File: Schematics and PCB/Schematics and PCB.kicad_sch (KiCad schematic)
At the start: 3 parts, among them J1 Magnetic Left, J2 Magnetic Right, U1 SN74AUC1G126DBVR

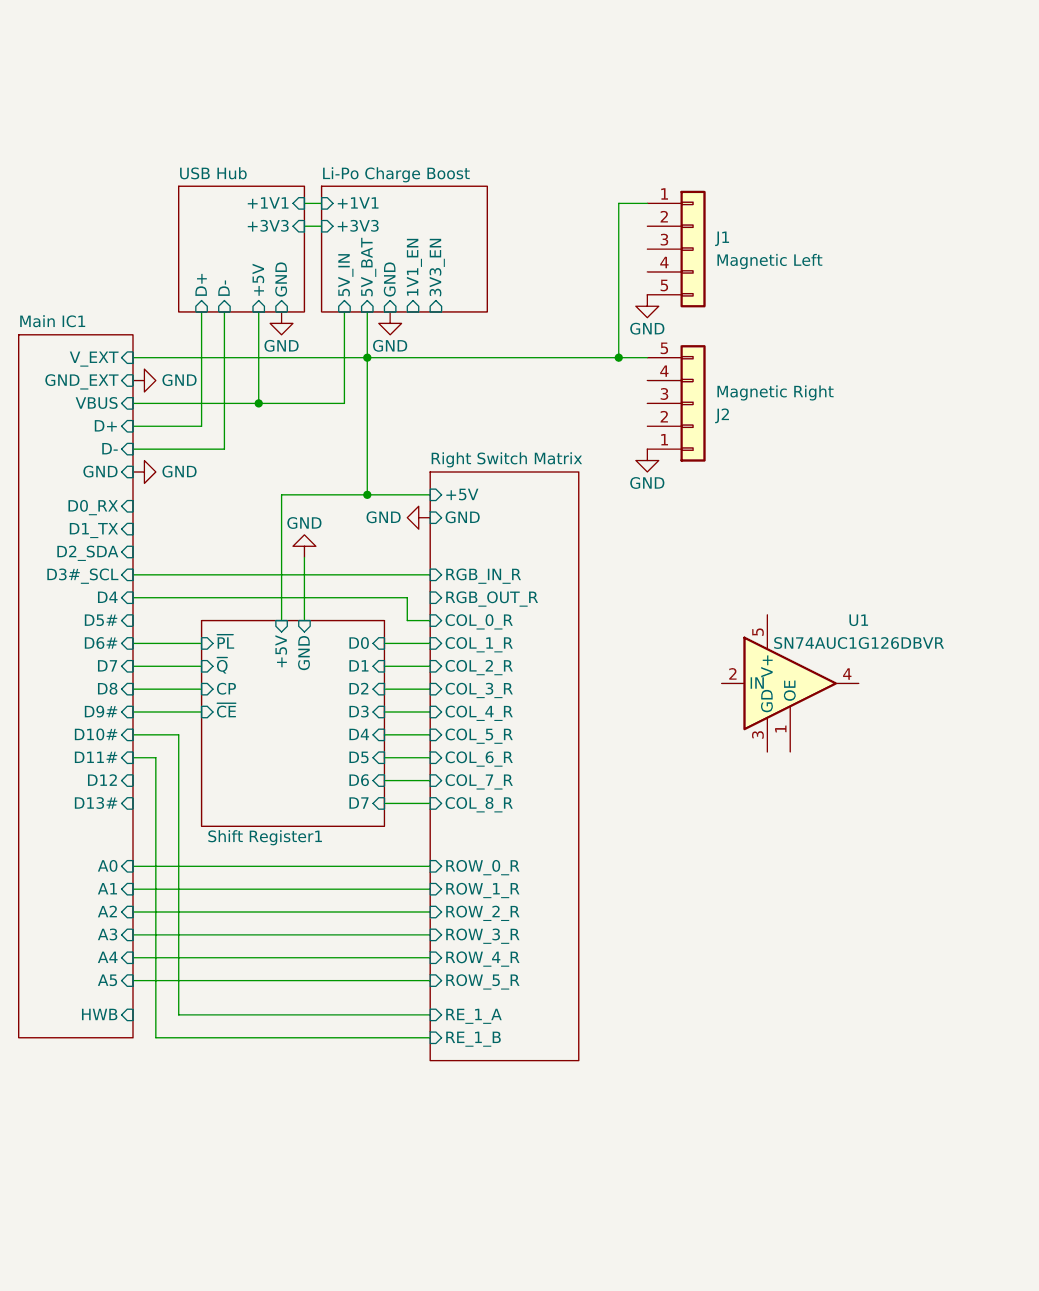
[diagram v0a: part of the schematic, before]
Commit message: Right layout created
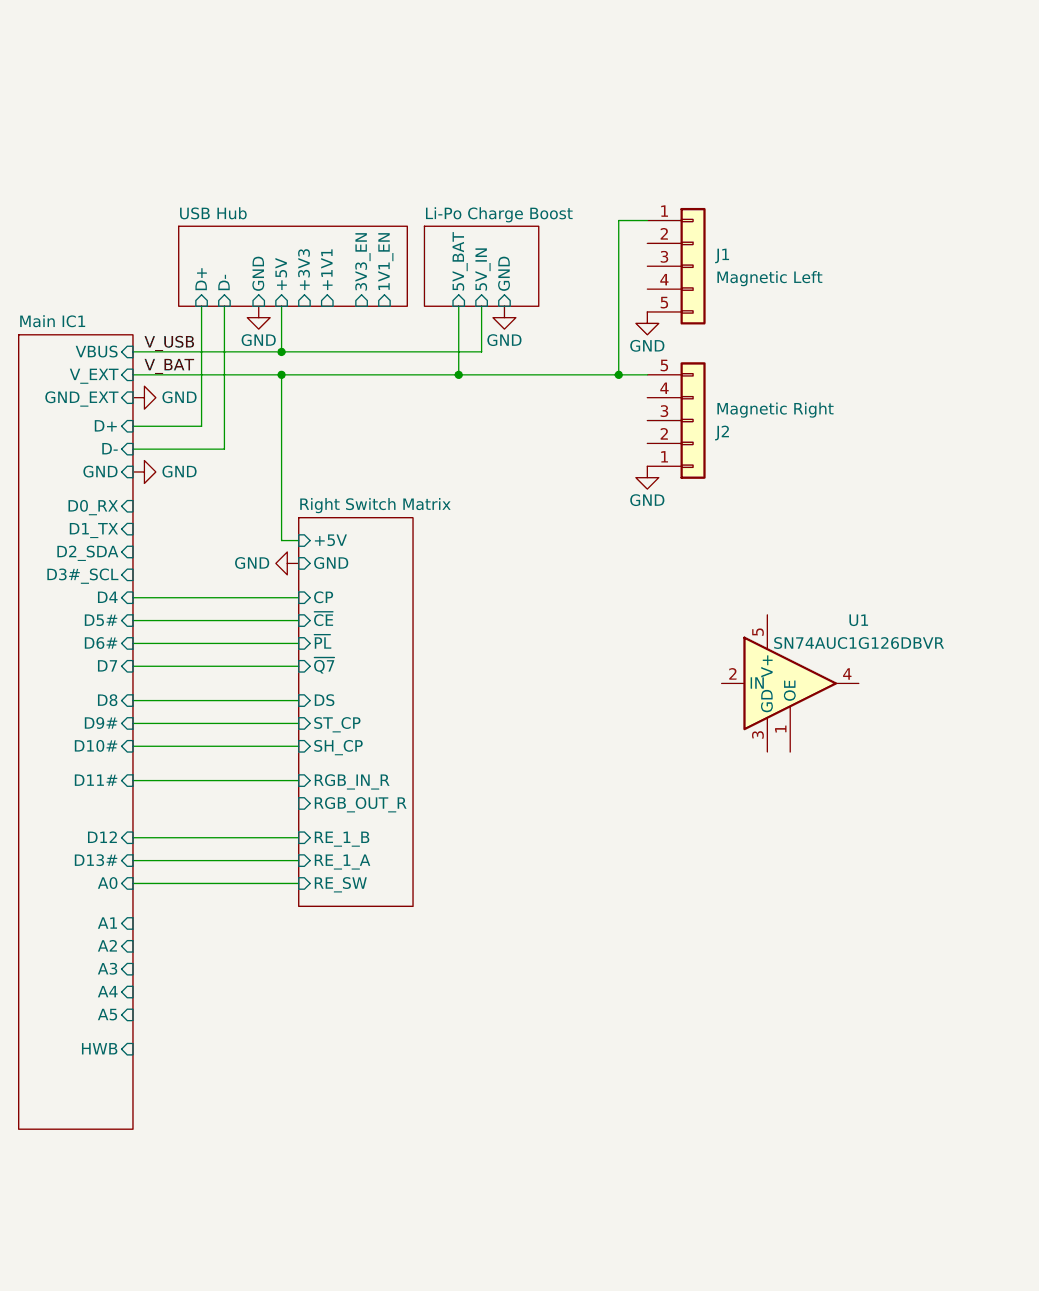
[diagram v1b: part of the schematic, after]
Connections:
- net Li-Po Charge Boost/5V_BAT renamed V_BAT
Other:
- removed sheet Shift Register1
- sheet Li-Po Charge Boost ports: added none; removed +1V1, +3V3, 1V1_EN, 3V3_EN
- sheet Right Switch Matrix ports: added CP, DS, RE_SW, SH_CP, ST_CP, ~{CE}, ~{PL}, ~{Q7}; removed COL_0_R, COL_1_R, COL_2_R, COL_3_R, COL_4_R, COL_5_R, COL_6_R, COL_7_R, COL_8_R, ROW_0_R, ROW_1_R, ROW_2_R, ROW_3_R, ROW_4_R, ROW_5_R
- sheet USB Hub ports: added 1V1_EN, 3V3_EN; removed none
- moved on the sheet: J1, J2
